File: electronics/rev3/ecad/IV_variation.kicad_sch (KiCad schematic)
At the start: 35 parts, among them Q5 TIP122, Q6 TIP127, U2 LMC6484A

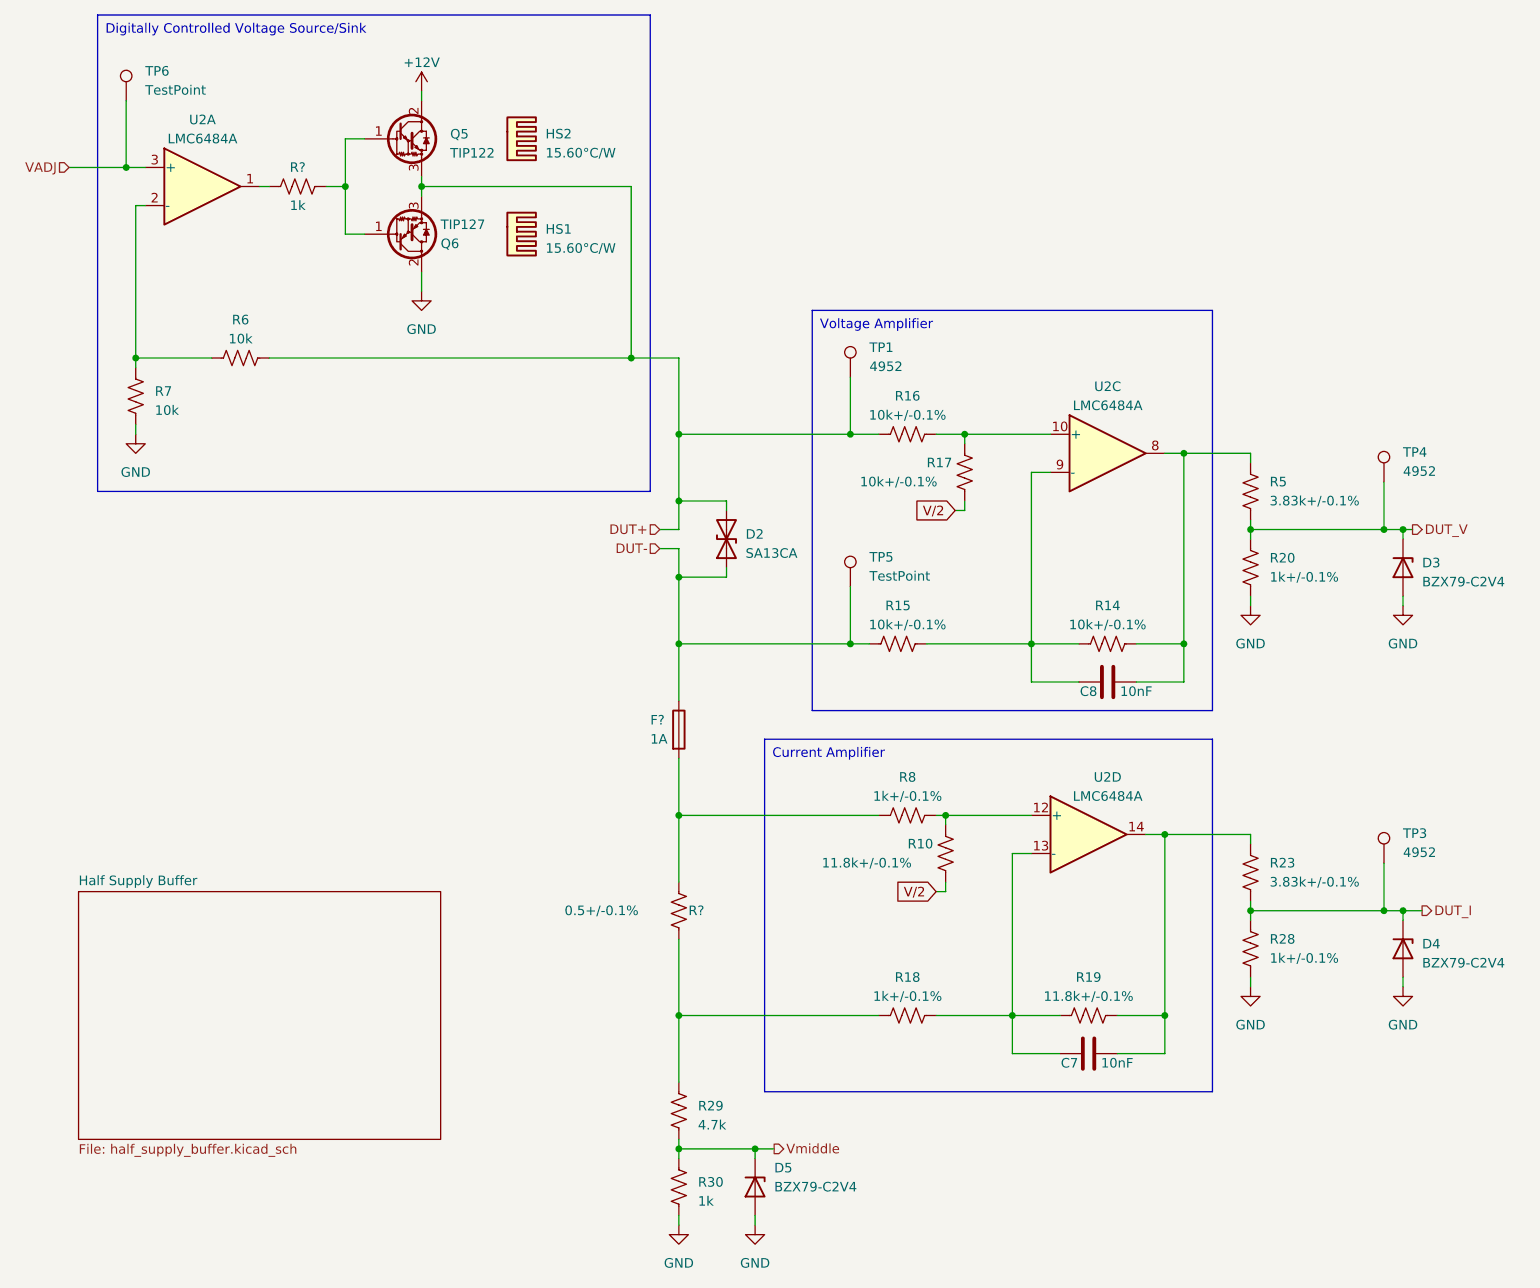
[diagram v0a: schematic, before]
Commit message: REV3 schematic
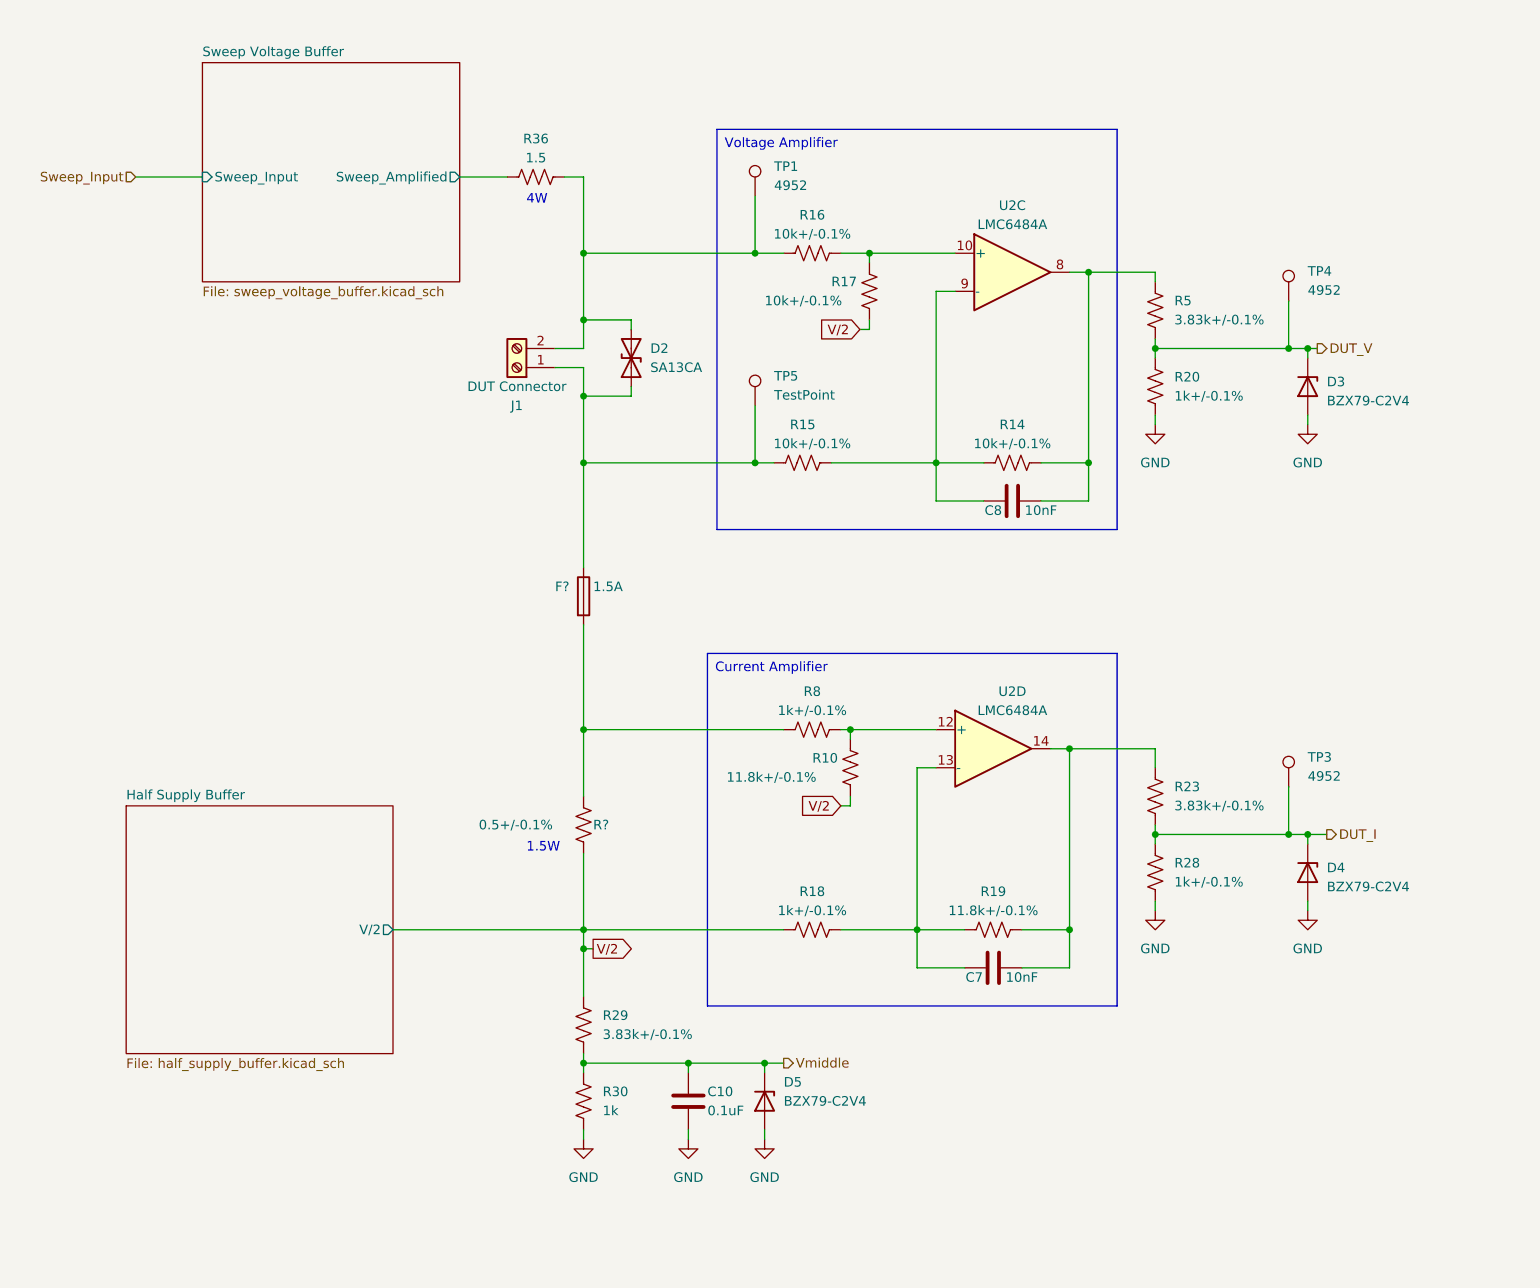
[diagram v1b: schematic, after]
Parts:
- removed HS1, HS2: 15.60°C/W, symbol Mechanical:Heatsink
- removed Q5: TIP122, Package_TO_SOT_THT:TO-220-3_Vertical, symbol Transistor_BJT:TIP122
- removed Q6: TIP127, Package_TO_SOT_THT:TO-220-3_Vertical, symbol Transistor_BJT:TIP127
- removed R6, R7: 10k, Resistor_THT:R_Axial_DIN0207_L6.3mm_D2.5mm_P7.62mm_Horizontal, symbol Device:R_US
- removed R?: 1k, Resistor_THT:R_Axial_DIN0207_L6.3mm_D2.5mm_P7.62mm_Horizontal, symbol Device:R_US
- removed TP6: TestPoint, TestPoint:TestPoint_THTPad_D2.5mm_Drill1.2mm, symbol Connector:TestPoint
- removed unit 1 of U2
- added C10: 0.1uF, Capacitor_THT:C_Disc_D6.0mm_W2.5mm_P5.00mm, symbol Device:C
- added J1: DUT Connector, TerminalBlock_Phoenix:TerminalBlock_Phoenix_MKDS-1,5-2-5.08_1x02_P5.08mm_Horizontal, symbol Connector:Screw_Terminal_01x02
- added R36: 1.5, Resistor_THT:R_Axial_DIN0207_L6.3mm_D2.5mm_P7.62mm_Horizontal, symbol Device:R_US
- C7, C8: footprint (none) -> Capacitor_THT:C_Disc_D6.0mm_W2.5mm_P5.00mm; Distributor Part # (none) -> BC2662CT-ND; Part # (none) -> K103K10X7RF5UH5; Unit Price (none) -> 0.22
- D2: Distributor Part # (none) -> SA13CACT-ND; Part # (none) -> SA13CA; Unit Price (none) -> 0.49
- D3, D4, D5: Distributor Part # (none) -> 1727-2115-1-ND; Part # (none) -> BZX79-C2V4,113; Unit Price (none) -> 0.16
- F?: value 1A -> 1.5A; Distributor Part # (none) -> 507-1893-1-ND; Part # (none) -> 0685T1500-01; Unit Price (none) -> 0.32
- R10, R19: Distributor Part # (none) -> 1712-YR1B11K8CCCT-ND; Part # (none) -> YR1B11K8CC; Unit Price (none) -> 0.63
- R14, R15, R16, R17: Distributor Part # (none) -> A105970CT-ND; Part # (none) -> YR1B10KCC; Unit Price (none) -> 0.63
- R18, R20, R28, R8: Distributor Part # (none) -> A105942CT-ND; Part # (none) -> YR1B1K0CC; Unit Price (none) -> 0.63
- R23, R5: Distributor Part # (none) -> 1712-YR1B3K83CCCT-ND; Part # (none) -> YR1B3K83CC; Unit Price (none) -> 0.63
- R29: value 4.7k -> 3.83k+/-0.1%
- R30: Distributor Part # (none) -> 13-MFR-25FRF52-1KCT-ND; Part # (none) -> MFR-25FRF52-1K; Unit Price (none) -> 0.1
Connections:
- net GND: now also C10.2
- net Vmiddle: now also C10.1
- net V/2: now also R18.1, R29.1, R?.2
- net DUT+: no longer names the net of D2.2 (A2), R16.1, TP1.1
- net DUT+: now also J1.2 (Pin_2), R36.2
- net DUT-: no longer names the net of D2.1 (A1), F?.1, R15.1, TP5.1
- net DUT-: now also J1.1 (Pin_1)
- new net Sweep Voltage Buffer/Sweep_Amplified: R36.1
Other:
- added sheet Sweep Voltage Buffer (sweep_voltage_buffer.kicad_sch)
- sheet Half Supply Buffer ports: added V/2; removed none
- note added: "1.5W"
- note added: "4W"
- moved on the sheet: C7, C8, D2, D3, D4, D5, F?, R10, R14, R15, R16, R17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
